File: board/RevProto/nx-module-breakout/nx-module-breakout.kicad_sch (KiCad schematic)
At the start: 8 parts, among them J1 Conn_02x15_Odd_Even, J2 DF40C-60DS-0.4V(51), J3 Conn_02x15_Odd_Even, J4 Conn_02x15_Odd_Even, J5 DF40C-60DS-0.4V(51), J6 SFV22R-2STE1HLF, J7 SFV22R-2STE1HLF, J8 Conn_02x06_Odd_Even

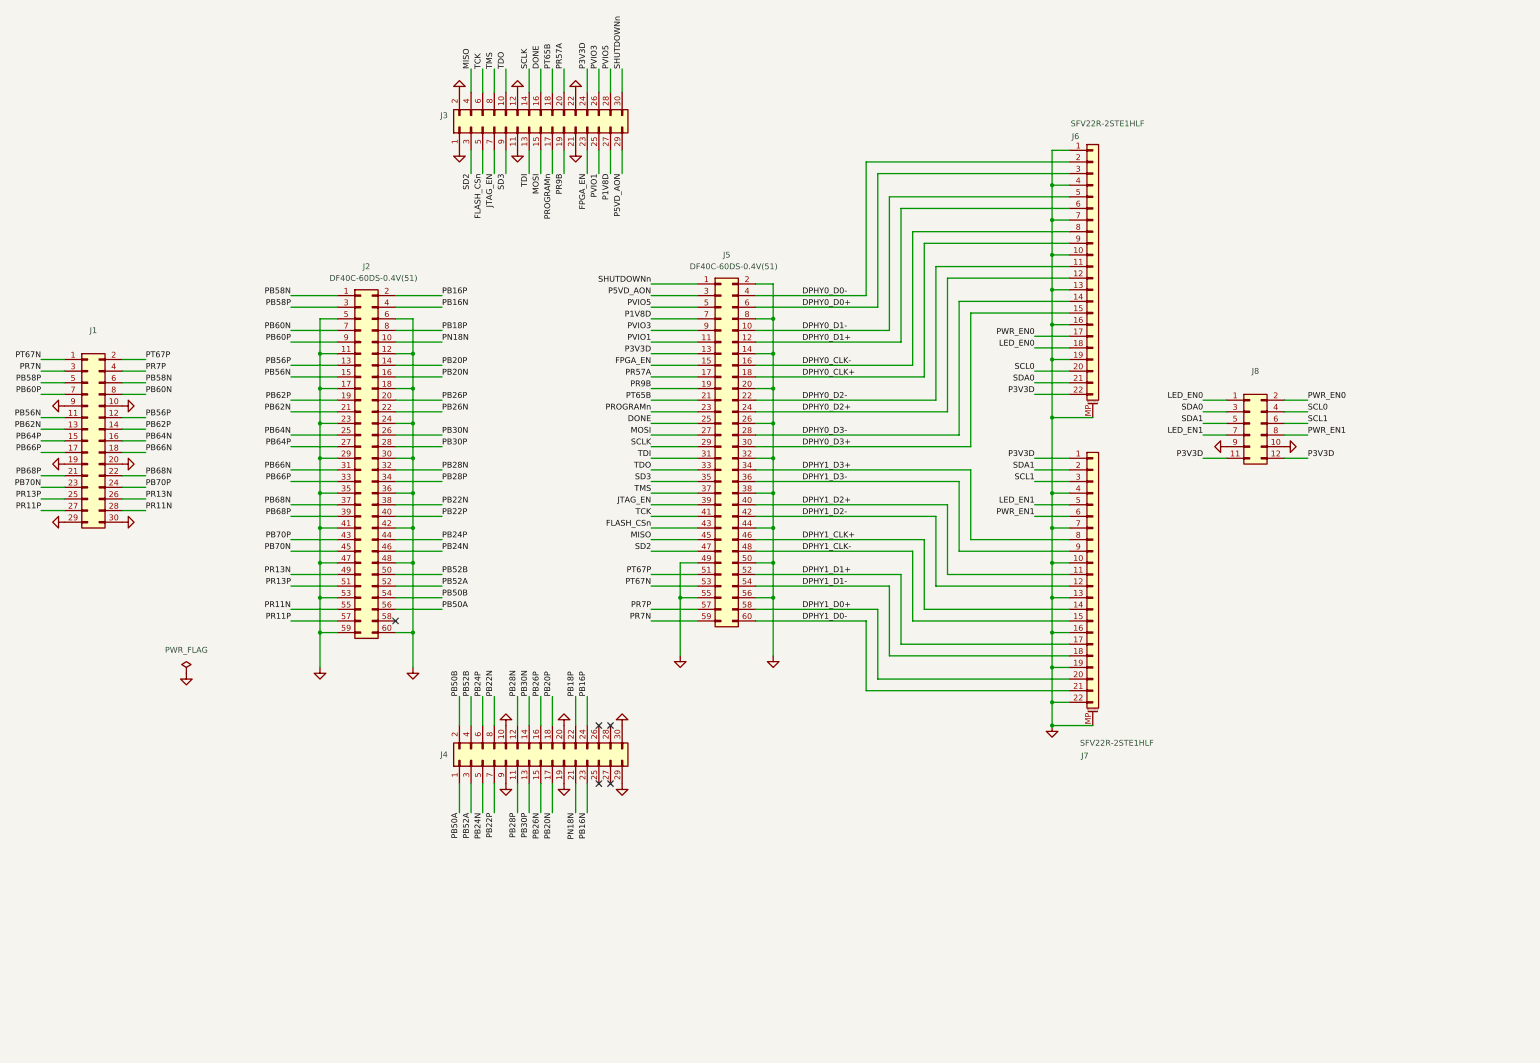
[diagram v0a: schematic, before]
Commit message: nx module breakout work in progress
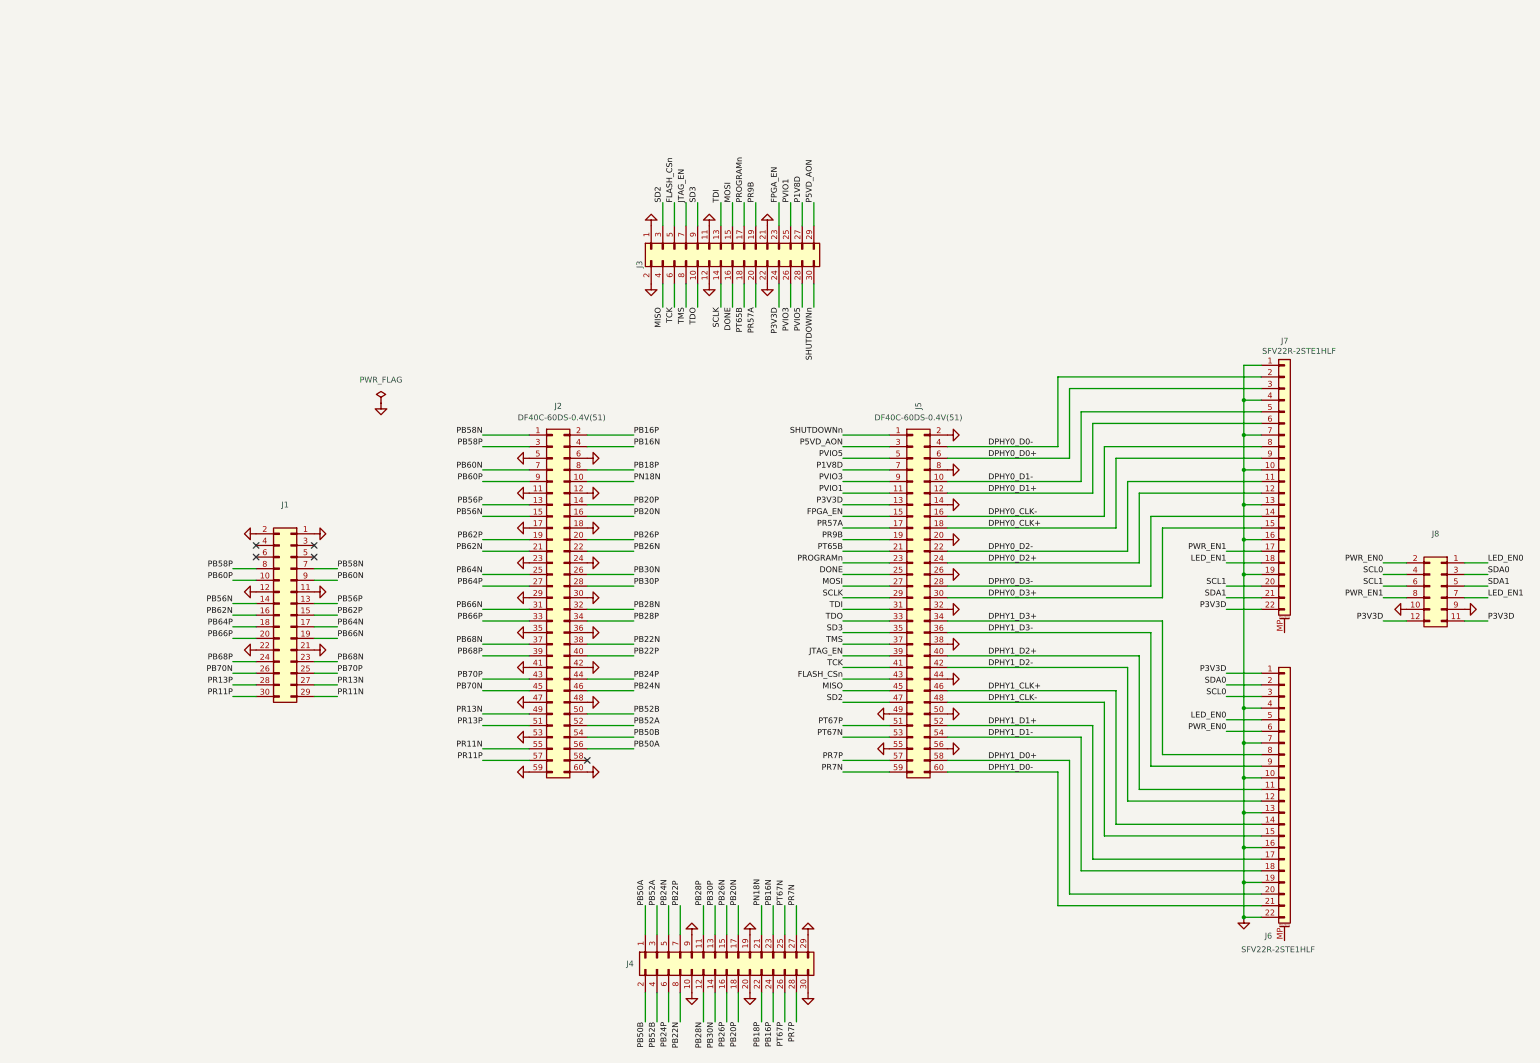
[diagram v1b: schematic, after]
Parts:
- J6, J7: footprint RP2350_60QFN_minimal:AMPHENOL_SFV22R-2STE1HLF -> CUSTOM:AMPHENOL_SFV22R-2STE1HLF
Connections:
- net DPHY0_CLK+: now also J7.9 (Pin_9); no longer J6.9 (Pin_9)
- net DPHY0_CLK-: now also J7.8 (Pin_8); no longer J6.8 (Pin_8)
- net DPHY0_D0+: now also J7.3 (Pin_3); no longer J6.3 (Pin_3)
- net DPHY0_D0-: now also J7.2 (Pin_2); no longer J6.2 (Pin_2)
- net DPHY0_D1+: now also J7.6 (Pin_6); no longer J6.6 (Pin_6)
- net DPHY0_D1-: now also J7.5 (Pin_5); no longer J6.5 (Pin_5)
- net DPHY0_D2+: now also J7.12 (Pin_12); no longer J6.12 (Pin_12)
- net DPHY0_D2-: now also J7.11 (Pin_11); no longer J6.11 (Pin_11)
- net DPHY0_D3+: now also J7.15 (Pin_15); no longer J6.15 (Pin_15)
- net DPHY0_D3-: now also J7.14 (Pin_14); no longer J6.14 (Pin_14)
- net DPHY1_CLK+: now also J6.14 (Pin_14); no longer J7.14 (Pin_14)
- net DPHY1_CLK-: now also J6.15 (Pin_15); no longer J7.15 (Pin_15)
- net DPHY1_D0+: now also J6.20 (Pin_20); no longer J7.20 (Pin_20)
- net DPHY1_D0-: now also J6.21 (Pin_21); no longer J7.21 (Pin_21)
- net DPHY1_D1+: now also J6.17 (Pin_17); no longer J7.17 (Pin_17)
- net DPHY1_D1-: now also J6.18 (Pin_18); no longer J7.18 (Pin_18)
- net DPHY1_D2+: now also J6.11 (Pin_11); no longer J7.11 (Pin_11)
- net DPHY1_D2-: now also J6.12 (Pin_12); no longer J7.12 (Pin_12)
- net DPHY1_D3+: now also J6.8 (Pin_8); no longer J7.8 (Pin_8)
- net DPHY1_D3-: now also J6.9 (Pin_9); no longer J7.9 (Pin_9)
- net GND: now also J1.1 (Pin_1), J1.11 (Pin_11), J1.12 (Pin_12), J1.2 (Pin_2), J1.21 (Pin_21), J1.22 (Pin_22), J6.22 (Pin_22), J7.1 (Pin_1); no longer J1.10 (Pin_10), J1.19 (Pin_19), J1.20 (Pin_20), J1.29 (Pin_29), J1.30 (Pin_30), J1.9 (Pin_9), J6.1 (Pin_1), J6.MP (MountPin), J7.22 (Pin_22), J7.MP (MountPin)
- net LED_EN0: now also J6.5 (Pin_5); no longer J6.18 (Pin_18)
- net LED_EN1: now also J7.18 (Pin_18); no longer J7.5 (Pin_5)
- net P3V3D: now also J6.1 (Pin_1), J7.22 (Pin_22); no longer J6.22 (Pin_22), J7.1 (Pin_1)
- net PB56N: now also J1.14 (Pin_14); no longer J1.11 (Pin_11)
- net PB56P: now also J1.13 (Pin_13); no longer J1.12 (Pin_12)
- net PB58N: now also J1.7 (Pin_7); no longer J1.6 (Pin_6)
- net PB58P: now also J1.8 (Pin_8); no longer J1.5 (Pin_5)
- net PB60N: now also J1.9 (Pin_9); no longer J1.8 (Pin_8)
- net PB60P: now also J1.10 (Pin_10); no longer J1.7 (Pin_7)
- net PB62N: now also J1.16 (Pin_16); no longer J1.13 (Pin_13)
- net PB62P: now also J1.15 (Pin_15); no longer J1.14 (Pin_14)
- net PB64N: now also J1.17 (Pin_17); no longer J1.16 (Pin_16)
- net PB64P: now also J1.18 (Pin_18); no longer J1.15 (Pin_15)
- net PB66N: now also J1.19 (Pin_19); no longer J1.18 (Pin_18)
- net PB66P: now also J1.20 (Pin_20); no longer J1.17 (Pin_17)
- net PB68N: now also J1.23 (Pin_23); no longer J1.22 (Pin_22)
- net PB68P: now also J1.24 (Pin_24); no longer J1.21 (Pin_21)
- net PB70N: now also J1.26 (Pin_26); no longer J1.23 (Pin_23)
- net PB70P: now also J1.25 (Pin_25); no longer J1.24 (Pin_24)
- net PR11N: now also J1.29 (Pin_29); no longer J1.28 (Pin_28)
- net PR11P: now also J1.30 (Pin_30); no longer J1.27 (Pin_27)
- net PR13N: now also J1.27 (Pin_27); no longer J1.26 (Pin_26)
- net PR13P: now also J1.28 (Pin_28); no longer J1.25 (Pin_25)
- net PR7N: now also J4.27 (Pin_27); no longer J1.3 (Pin_3)
- net PR7P: now also J4.28 (Pin_28); no longer J1.4 (Pin_4)
- net PT67N: now also J4.25 (Pin_25); no longer J1.1 (Pin_1)
- net PT67P: now also J4.26 (Pin_26); no longer J1.2 (Pin_2)
- net PWR_EN0: now also J6.6 (Pin_6); no longer J6.17 (Pin_17)
- net PWR_EN1: now also J7.17 (Pin_17); no longer J7.6 (Pin_6)
- net SCL0: now also J6.3 (Pin_3); no longer J6.20 (Pin_20)
- net SCL1: now also J7.20 (Pin_20); no longer J7.3 (Pin_3)
- net SDA0: now also J6.2 (Pin_2); no longer J6.21 (Pin_21)
- net SDA1: now also J7.21 (Pin_21); no longer J7.2 (Pin_2)
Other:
- moved on the sheet: J1, J2, J3, J4, J5, J6, J7, J8
